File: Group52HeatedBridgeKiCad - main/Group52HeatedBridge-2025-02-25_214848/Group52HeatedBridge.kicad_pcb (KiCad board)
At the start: 2 copper layers, 100 x 100 mm, 24 parts, among them J1 UART, J10 TempSensorAirLED, J2 RainSensor, J3 TemperatureSurface, J4 TemperatureAir, J5 JTAG, J6 TempSensorSurfaceLED, J7 RainSensor LED, J8 EN_BUTTON, J9 BOOT_BUTTON, U1 ESP32-WROOM-32, U2 XL1509-3.3

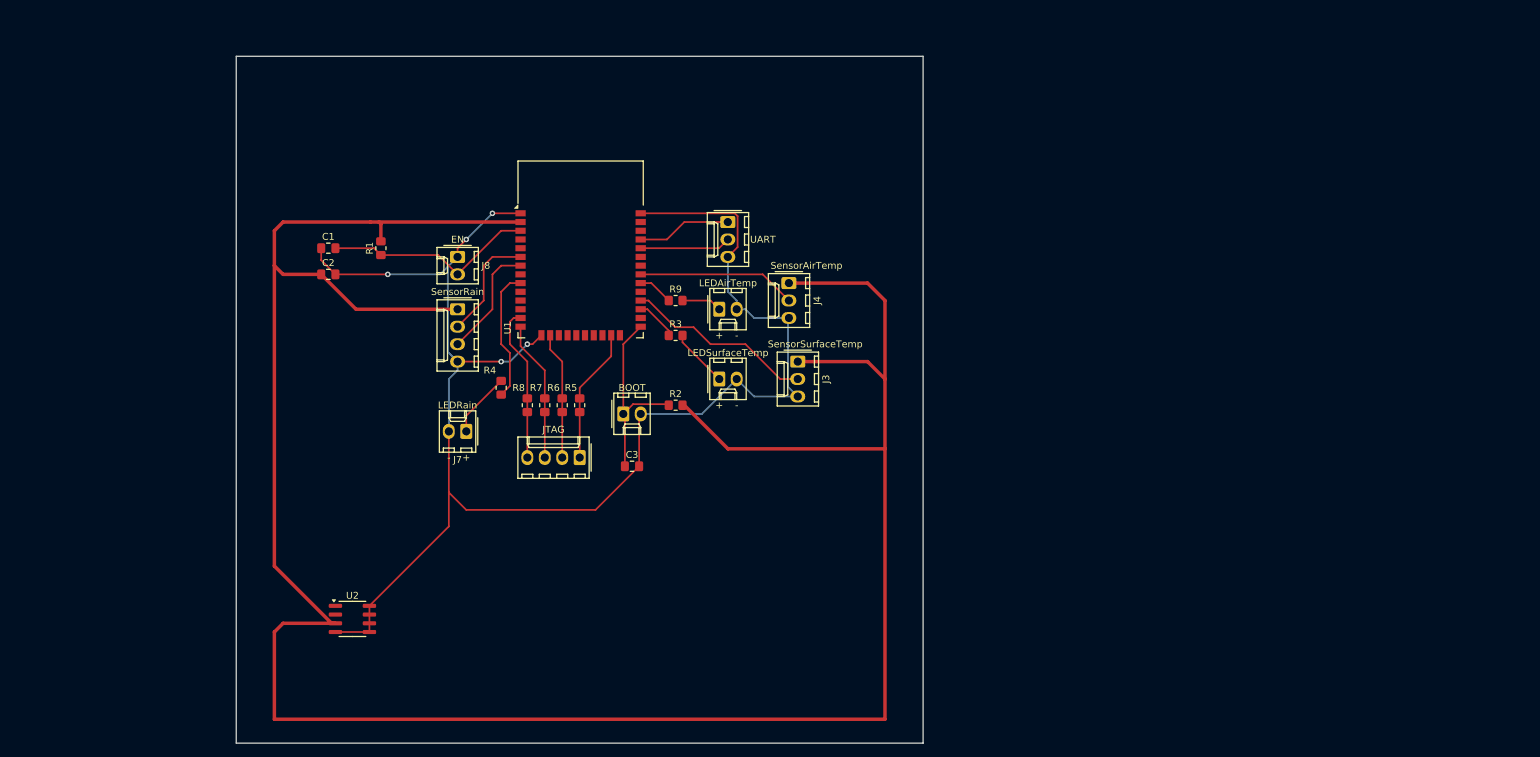
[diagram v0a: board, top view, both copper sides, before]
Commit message: B Revert "resized schematic and cleaned up"
This reverts commit bab35e5b8986f5439bb45f55d315508e4487ff8d.

reverted auto save file
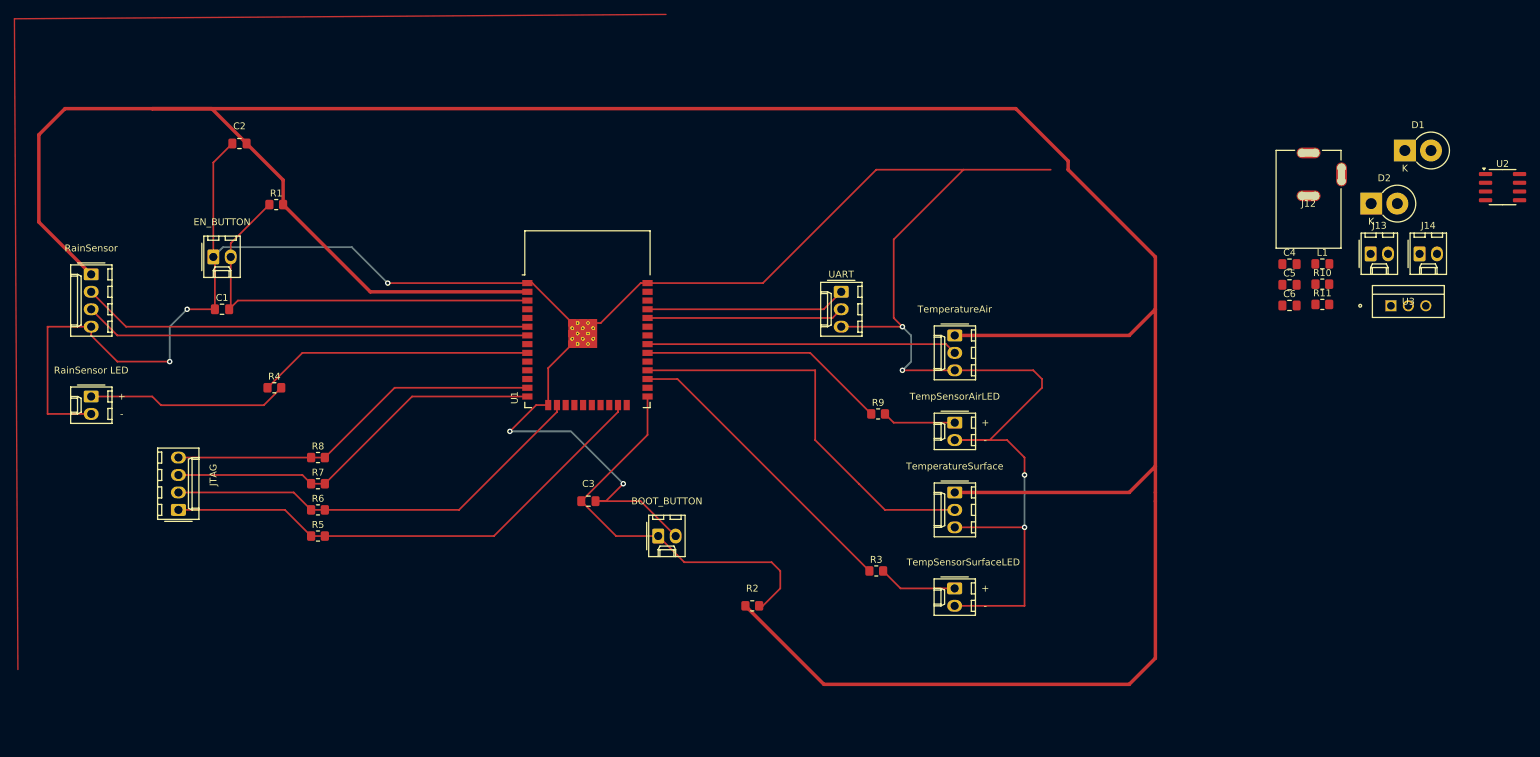
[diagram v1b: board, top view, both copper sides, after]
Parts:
- added C4: 470uf, Capacitor_SMD:C_0805_2012Metric_Pad1.18x1.45mm_HandSolder, F.Cu at (249.4, 73.4)
- added C5: 330uf, Capacitor_SMD:C_0805_2012Metric_Pad1.18x1.45mm_HandSolder, F.Cu at (249.4, 76.4)
- added C6: 1uf, Capacitor_SMD:C_0805_2012Metric_Pad1.18x1.45mm_HandSolder, F.Cu at (249.4, 79.5)
- added D1: 1N5820, Diode_THT:D_DO-201AD_P3.81mm_Vertical_KathodeUp, F.Cu at (266.2, 56.9)
- added D2: 1N5820, Diode_THT:D_DO-201AD_P3.81mm_Vertical_KathodeUp, F.Cu at (261.3, 64.6)
- added J12: 54-00166, footprints_barrel:CONN3_54-00166_TEN, F.Cu at (252.2, 57.2)
- added J13: Heater1, Connector_Molex:Molex_KK-254_AE-6410-02A_1x02_P2.54mm_Vertical, F.Cu at (261.2, 71.9)
- added J14: Heater2, Connector_Molex:Molex_KK-254_AE-6410-02A_1x02_P2.54mm_Vertical, F.Cu at (268.3, 71.9)
- added L1: 47uh, Inductor_SMD:L_0805_2012Metric_Pad1.15x1.40mm_HandSolder, F.Cu at (254.2, 73.4)
- added R10: 10, Resistor_SMD:R_0805_2012Metric_Pad1.20x1.40mm_HandSolder, F.Cu at (254.2, 76.4)
- added R11: 10k, Resistor_SMD:R_0805_2012Metric_Pad1.20x1.40mm_HandSolder, F.Cu at (254.2, 79.3)
- added U3: IRLZ44NPBF, footprints:PG-TO220-3_INF, F.Cu at (264.2, 79.5)
- moved U2 178.9 mm to (280.4, 62.2)
- moved J5 58.9 mm to (87.6, 109.2), turned to 90 degrees
- moved J7 54.8 mm to (74.9, 92.7), turned to -90 degrees
- moved J2 53.6 mm to (74.9, 74.9)
- moved J6 45.9 mm to (200.6, 120.7), turned to -90 degrees
- moved R3 45.0 mm to (189.2, 118.1)
- moved R5 42.6 mm to (108.0, 113.0), turned to 0 degrees
- moved R6 38.7 mm to (108.0, 109.2), turned to 0 degrees
- moved J10 38.1 mm to (200.7, 96.5), turned to -90 degrees
- moved J8 35.6 mm to (92.7, 72.4), turned to 0 degrees
- moved R7 34.9 mm to (108.0, 105.4), turned to 0 degrees
- moved R9 33.8 mm to (189.5, 95.2)
- moved R4 33.0 mm to (101.6, 91.4), turned to 0 degrees
- moved R8 31.4 mm to (108.0, 101.6), turned to 0 degrees
- moved R2 31.3 mm to (171.2, 123.2), turned to 180 degrees
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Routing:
- net GND: track 229.4 -> 404.5 mm, vias 5 -> 9
- net +3.3V: track 362.6 -> 451.1 mm
- net /MTDO: track 19.7 -> 74.1 mm
- net /DigitalRain: track 16.4 -> 65.6 mm
- net /AnalogRain: track 16.9 -> 65.1 mm
- net /MTCK: track 18.5 -> 63.1 mm
- net /GPIOTempSurfaceLED: track 6.07 -> 43.9 mm
- net /MTDI: track 20.5 -> 56.6 mm
- net /MTMS: track 22.6 -> 55.0 mm
- net /GPIOTempSurface: track 27.6 -> 59.1 mm
- net /GPIOTempAirLED: track 5.13 -> 36.3 mm
- net /EN: track 31.2 -> 61.6 mm
- net /BOOT: track 28.7 -> 59.1 mm
- net /GPIOTempAir: track 23.1 -> 45.3 mm
- net /GPIORainLED: track 19.4 -> 39.9 mm
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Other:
- board size 100 x 100 mm -> 5.8 x 6.2 mm
